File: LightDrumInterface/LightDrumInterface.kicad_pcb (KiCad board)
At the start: 2 copper layers, 108 x 83 mm, 74 parts, among them J1 MIDI-IN, J3 DEBUG-CONN, J4 PWR-CONN, J5 MIDI-OUT, J6 0541323662, Q1 NX6008NBKWX, Q2 NX6008NBKWX, Q3 NX6008NBKWX, Q4 NX6008NBKWX, SW1 RESET-SW, U1 STP16CP05, U2 TPL0401B-10-Q1, U3 PC817, U4 74AUP2G04

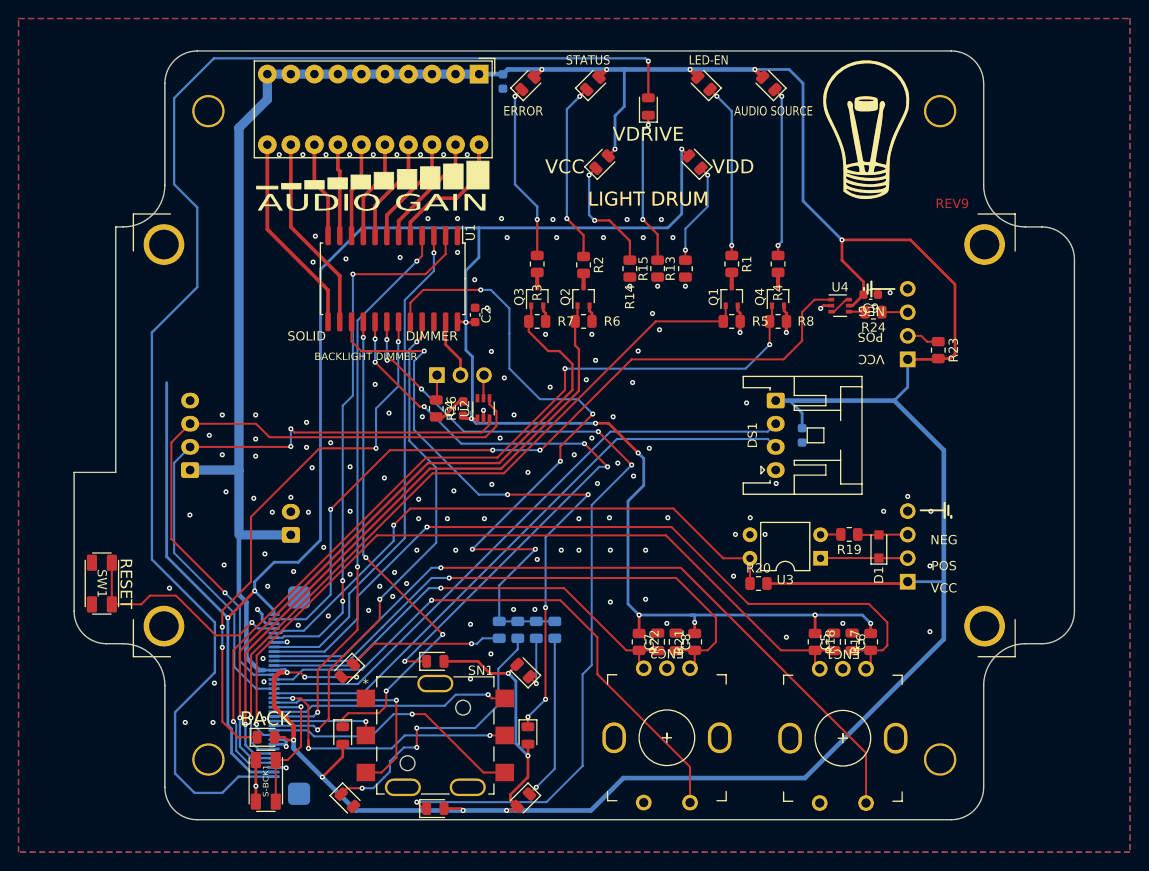
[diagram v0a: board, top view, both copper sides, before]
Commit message: Main and Interface PCBs locked - REV9
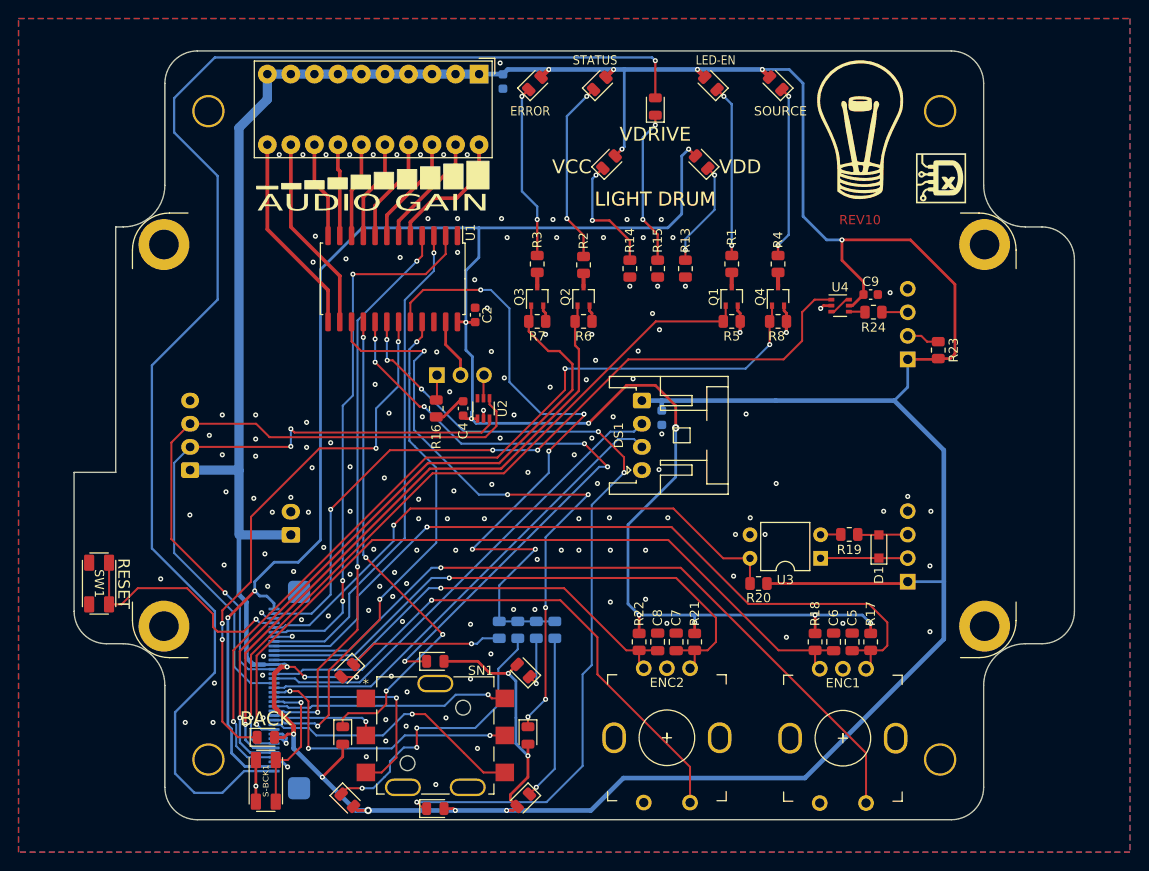
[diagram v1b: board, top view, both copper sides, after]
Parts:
- added G***: LOGO, Daxxn_Logos_Art:Daxxn_Logo_S, F.Cu at (112.8, 38.2)
- J4: footprint Connector_JST:JST_XA_B02B-XASK-1_1x02_P2.50mm_Vertical -> Daxxn_Connectors:JST_XH_B2B-XH-A_Vertical
- moved C1 15.3 mm to (82.6, 64.1)
- moved DS1 14.5 mm to (80.5, 66.0)
- moved D-AUDIO-SEL1 0.75 mm to (94.9, 28.0)
- moved D-DBG1 0.75 mm to (68.9, 28.0)
- moved D-STA1 0.75 mm to (75.9, 28.0)
- moved D-STRIP-EN1 0.75 mm to (87.9, 28.0)
- moved D-VCC1 0.75 mm to (76.9, 36.5)
- moved D-VDD1 0.75 mm to (86.9, 36.5)
- moved D-VDRIVE1 0.75 mm to (81.9, 30.5)
- moved G*** 0.65 mm to (104.0, 33.0) (x2)
- moved J6 0.60 mm to (40.7, 93.5)
- moved SW1 0.30 mm to (21.9, 82.0)
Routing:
- net VDD: track 241.0 -> 224.4 mm
- net /SCR-RX: track 65.9 -> 51.2 mm
- net /SCR-TX: track 65.8 -> 51.5 mm
- net VCC: track 415.4 -> 428.0 mm, vias 15 -> 16
- net Vdrive: track 149.9 -> 152.8 mm
- net /~{RESET}: track 25.0 -> 26.5 mm
- net /ENC1-B: track 85.0 -> 84.1 mm
- net Net-(D-MD1-Pad1): track 90.8 -> 90.1 mm
- net /DIAG-STATUS: track 70.6 -> 70.0 mm
- net /AUDIO-SRC-IND: track 92.8 -> 92.3 mm
- net /DIAG-DEBUG: track 73.9 -> 73.4 mm
- net GND: vias 135 -> 153
- net (no net): vias 5 -> 0
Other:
- board text added: "REV10"
- board text added: "SOURCE"
- board text added: "VCC PWR"
- board text removed: "AUDIO SOURCE"
- board text removed: "REV9"
